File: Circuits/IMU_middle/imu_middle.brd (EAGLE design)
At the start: 16.4 x 16 mm, 11 parts, among them U1 LSM9DS1

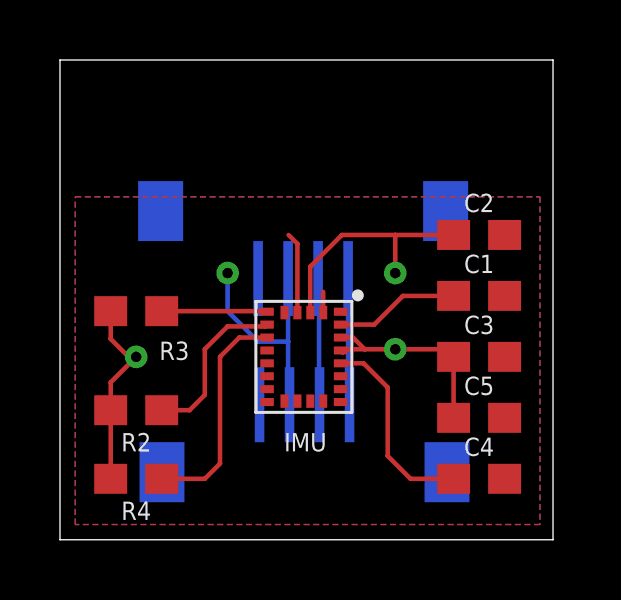
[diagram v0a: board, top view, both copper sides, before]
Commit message: ghetto board design
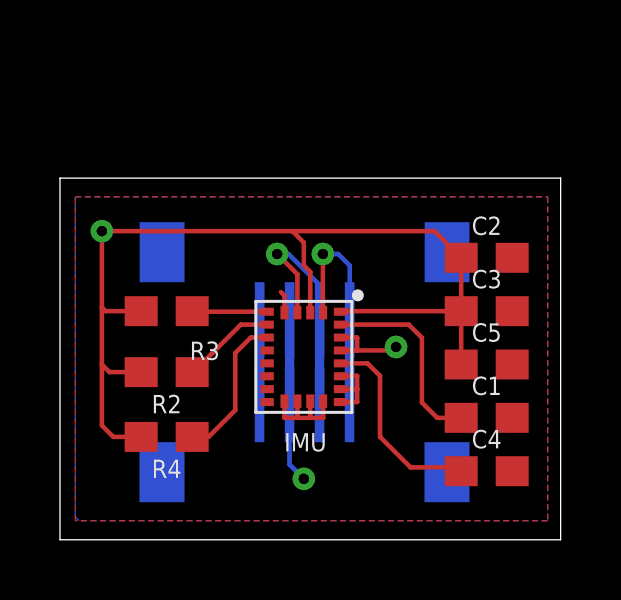
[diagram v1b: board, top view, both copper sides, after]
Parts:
- moved C1 4.07 mm to (53.6, 33.0)
- moved C5 1.80 mm to (53.6, 34.8)
- moved R4 1.73 mm to (42.9, 32.4)
- moved R2 1.63 mm to (42.9, 34.5)
- moved C3 1.55 mm to (53.6, 36.6)
- moved U$2 1.37 mm to (46.0, 37.5)
- moved R3 1.02 mm to (42.9, 36.6)
- moved C2 0.80 mm to (53.6, 38.4)
- moved C4 0.36 mm to (53.6, 31.2)
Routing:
- net VCC: track 21.4 -> 39.3 mm, vias 3 -> 2
- net GND: track 7.50 -> 12.3 mm
- net SCL: track 4.09 -> 7.65 mm, vias 0 -> 1
- net CS_M: track 7.55 -> 4.98 mm
- net CS_A/G: track 5.59 -> 3.15 mm
- net C1: track 4.16 -> 6.57 mm
- net SDA: track 5.84 -> 8.07 mm, vias 0 -> 1
- net SA1: track 3.52 -> 2.50 mm
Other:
- board size 16.4 x 16 mm -> 16.7 x 12.1 mm
